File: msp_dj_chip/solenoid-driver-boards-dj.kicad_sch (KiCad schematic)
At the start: 0 parts

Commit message: updated changes
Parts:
- added C19: C_Small, symbol Device:C_Small
- added Q1: NMOS, symbol Simulation_SPICE:NMOS
- added R48: 30K, symbol Device:R_Small
- added R49: 500, symbol Device:R_Small
- added R50: 1K2, symbol Device:R_Small
- added R51, R52: 1, symbol Device:R_Small
- added R53: 0, symbol Device:R_Small
- added TP2, TP3, TP4, TP5, TP6: TestPoint, symbol Connector:TestPoint
- added U16: ${SIM.PARAMS}, symbol Simulation_SPICE:OPAMP
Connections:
- new net: R48.2, R49.1, TP2.1, U16.1 (+)
- new net: C19.2, Q1.2 (G), R51.2, R53.1, TP5.1
- new net: Q1.1 (D), TP6.1
- new net: C19.1, R53.2, U16.5
- new net: Q1.3 (S), R50.1, R50.2, R52.2, TP3.1, TP4.1, U16.2 (-)
- new net +24V: U16.3 (V+)
- new net GND: R49.2, R51.1, R52.1, U16.4 (V-)

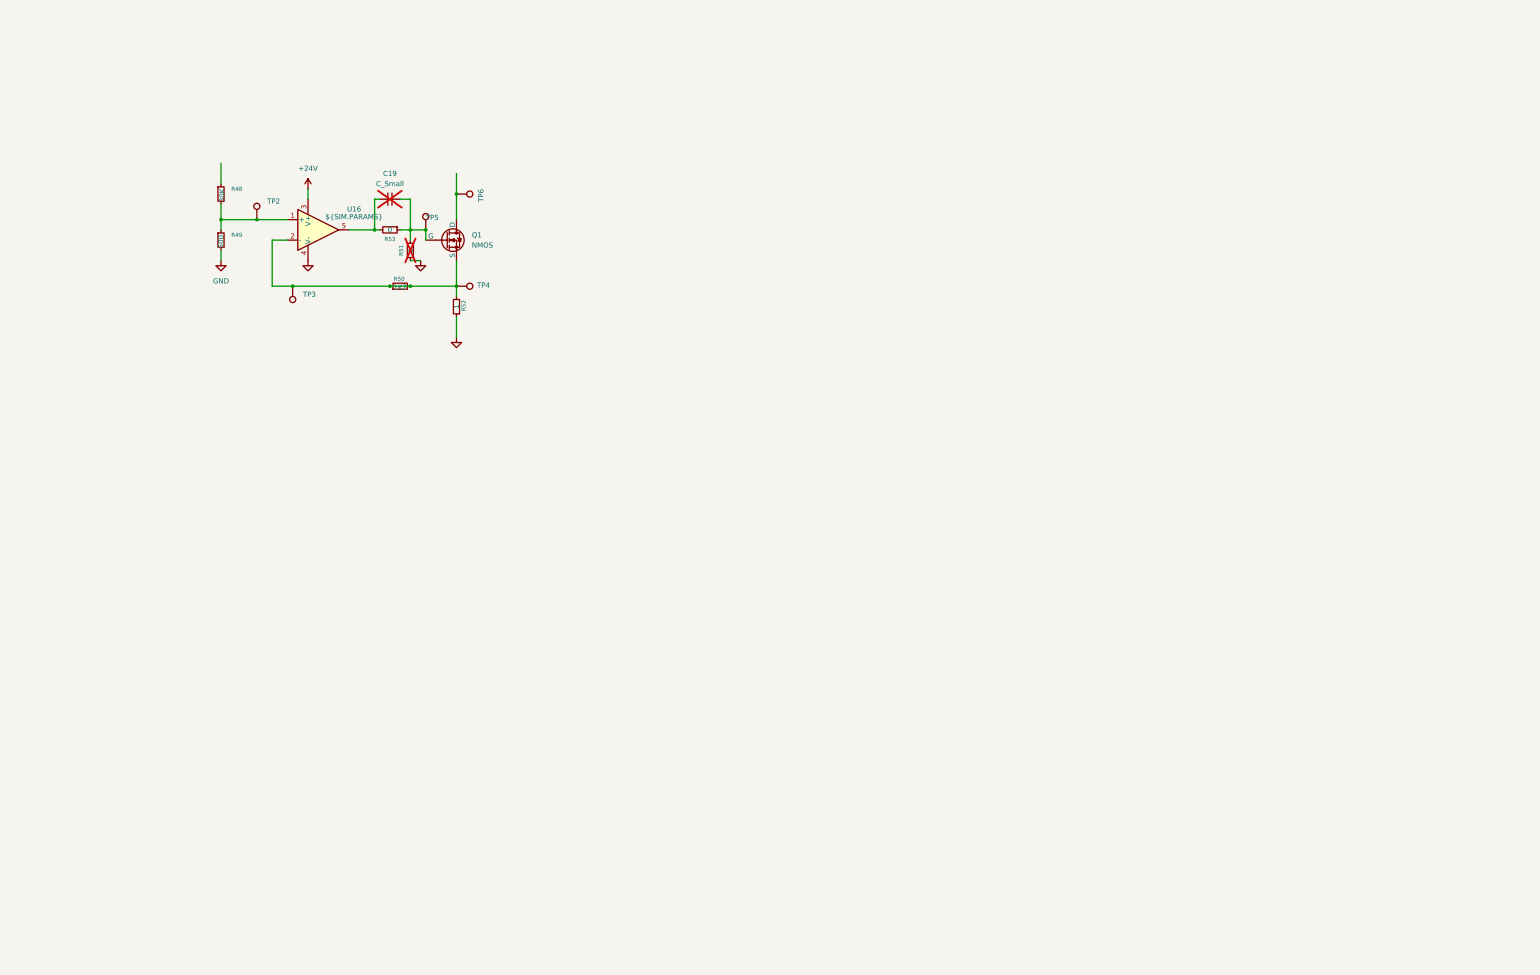
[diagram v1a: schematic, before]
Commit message: SOL-DRIVER-SHEET-ADDED
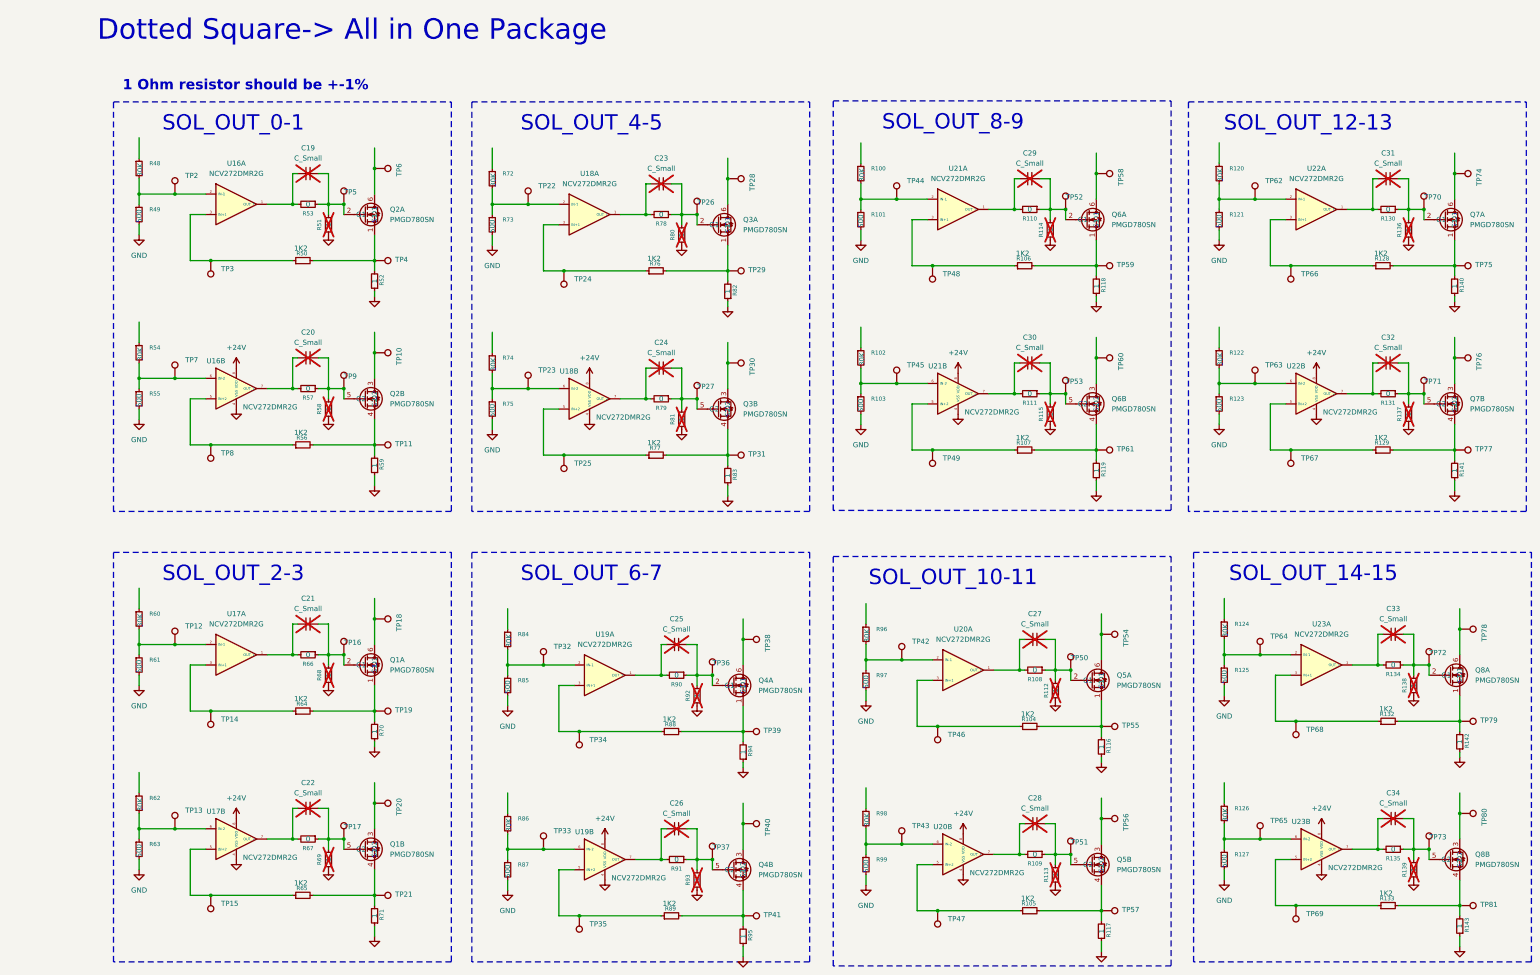
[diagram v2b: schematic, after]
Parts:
- removed Q1: NMOS, symbol Simulation_SPICE:NMOS
- removed U16: ${SIM.PARAMS}, symbol Simulation_SPICE:OPAMP
- added C20, C21, C22, C23, C24, C25, C26, C27, C28, C29, C30, C31, C32, C33, C34: C_Small, symbol Device:C_Small
- added Q1, Q2, Q3, Q4, Q5, Q6, Q7, Q8: PMGD780SN, project_footprints:PMGD780SN, symbol Project_Symbols:2N-Channel_MOSFET
- added R100, R102, R120, R122, R124, R126, R54, R60, R62, R72, R74, R84, R86, R96, R98: 30K, symbol Device:R_Small
- added R101, R103, R121, R123, R125, R127, R55, R61, R63, R73, R75, R85, R87, R97, R99: 500, symbol Device:R_Small
- added R104, R105, R106, R107, R128, R129, R132, R133, R56, R64, R65, R76, R77, R88, R89: 1K2, symbol Device:R_Small
- added R108, R109, R110, R111, R130, R131, R134, R135, R57, R66, R67, R78, R79, R90, R91: 0, symbol Device:R_Small
- added R112, R113, R114, R115, R116, R117, R118, R119, R136, R137, R138, R139, R140, R141, R142, R143, R58, R59, R68, R69, R70, R71, R80, R81, R82, R83, R92, R93, R94, R95: 1, symbol Device:R_Small
- added TP10, TP11, TP12, TP13, TP14, TP15, TP16, TP17, TP18, TP19, TP20, TP21, TP22, TP23, TP24, TP25, TP26, TP27, TP28, TP29, TP30, TP31, TP32, TP33, TP34, TP35, TP36, TP37, TP38, TP39, TP40, TP41, TP42, TP43, TP44, TP45, TP46, TP47, TP48, TP49, TP50, TP51, TP52, TP53, TP54, TP55, TP56, TP57, TP58, TP59, TP60, TP61, TP62, TP63, TP64, TP65, TP66, TP67, TP68, TP69, TP7, TP70, TP71, TP72, TP73, TP74, TP75, TP76, TP77, TP78, TP79, TP8, TP80, TP81, TP9: TestPoint, symbol Connector:TestPoint
- added U16, U17, U18, U19, U20, U21, U22, U23: NCV272DMR2G, Package_SO:MSOP-8_3x3mm_P0.65mm, symbol Project_Symbols:OpAmp_NCV272
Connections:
- net +24V: now also U16.8 (VDD), U17.8 (VDD), U18.8 (VDD), U19.8 (VDD), U20.8 (VDD), U21.8 (VDD), U22.8 (VDD), U23.8 (VDD)
- net GND: now also R101.2, R103.2, R112.1, R113.1, R114.1, R115.1, R116.1, R117.1, R118.1, R119.1, R121.2, R123.2, R125.2, R127.2, R136.1, R137.1, R138.1, R139.1, R140.1, R141.1, R142.1, R143.1, R55.2, R58.1, R59.1, R61.2, R63.2, R68.1, R69.1, R70.1, R71.1, R73.2, R75.2, R80.1, R81.1, R82.1, R83.1, R85.2, R87.2, R92.1, R93.1, R94.1, R95.1, R97.2, R99.2, U16.4 (VSS), U17.4 (VSS), U18.4 (VSS), U19.4 (VSS), U20.4 (VSS), U21.4 (VSS), U22.4 (VSS), U23.4 (VSS)
- net at R48.2, R49.1, TP2.1: now also U16.2 (IN-1)
- net at C19.2, R51.2, R53.1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: now also Q2.2 (G1)
- net at TP6.1: now also Q2.6 (D1)
- net at C19.1, R53.2: now also U16.1 (OUT_1)
- net at R50.2, R52.2, TP4.1: now also Q2.1 (S1); no longer R50.1, TP3.1
- new net: C23.2, Q3.2 (G1), R78.1, R80.2, TP26.1
- new net: R72.2, R73.1, TP22.1, U18.2 (IN-1)
- new net: R60.2, R61.1, TP12.1, U17.2 (IN-1)
- new net: C21.2, Q1.2 (G1), R66.1, R68.2, TP16.1
- new net: C21.1, R66.2, U17.1 (OUT_1)
- new net: Q4.4 (S2), R89.2, R95.2, TP41.1
- new net: R96.2, R97.1, TP42.1, U20.2 (IN-1)
- new net: C26.2, Q4.5 (G2), R91.1, R93.2, TP37.1
- new net: R128.1, TP66.1, U22.3 (IN+1)
- new net: C25.2, Q4.2 (G1), R90.1, R92.2, TP36.1
- new net: Q3.6 (D1), TP28.1
- new net: R74.2, R75.1, TP23.1, U18.6 (IN-2)
- new net: Q1.6 (D1), TP18.1
- new net: C27.2, Q5.2 (G1), R108.1, R112.2, TP50.1
- new net: C27.1, R108.2, U20.1 (OUT_1)
- new net: R129.1, TP67.1, U22.5 (IN+2)
- new net: Q7.4 (S2), R129.2, R141.2, TP77.1
- new net: R105.1, TP47.1, U20.5 (IN+2)
- new net: Q8.1 (S1), R132.2, R142.2, TP79.1
- new net: C33.2, Q8.2 (G1), R134.1, R138.2, TP72.1
- new net: Q8.6 (D1), TP78.1
- new net: R126.2, R127.1, TP65.1, U23.6 (IN-2)
- new net: C25.1, R90.2, U19.1 (OUT_1)
- new net: R133.1, TP69.1, U23.5 (IN+2)
- new net: C34.1, R135.2, U23.7 (OUT_2)
- new net: R84.2, R85.1, TP32.1, U19.2 (IN-1)
- new net: R88.1, TP34.1, U19.3 (IN+1)
- new net: R89.1, TP35.1, U19.5 (IN+2)
- new net: R86.2, R87.1, TP33.1, U19.6 (IN-2)
- new net: C26.1, R91.2, U19.7 (OUT_2)
- new net: C24.1, R79.2, U18.7 (OUT_2)
- new net: C24.2, Q3.5 (G2), R79.1, R81.2, TP27.1
- new net: R107.1, TP49.1, U21.5 (IN+2)
- new net: R102.2, R103.1, TP45.1, U21.6 (IN-2)
- new net: C30.1, R111.2, U21.7 (OUT_2)
- new net: R76.1, TP24.1, U18.3 (IN+1)
- new net: C22.1, R67.2, U17.7 (OUT_2)
- new net: C22.2, Q1.5 (G2), R67.1, R69.2, TP17.1
- new net: C20.2, Q2.5 (G2), R57.1, R58.2, TP9.1
- new net: C20.1, R57.2, U16.7 (OUT_2)
- new net: Q3.1 (S1), R76.2, R82.2, TP29.1
- new net: Q8.3 (D2), TP80.1
- new net: Q8.4 (S2), R133.2, R143.2, TP81.1
- new net: C34.2, Q8.5 (G2), R135.1, R139.2, TP73.1
- new net: Q6.3 (D2), TP60.1
- new net: R104.1, TP46.1, U20.3 (IN+1)
- new net: C23.1, R78.2, U18.1 (OUT_1)
- new net: Q4.1 (S1), R88.2, R94.2, TP39.1
- new net: Q4.6 (D1), TP38.1
- new net: Q5.6 (D1), TP54.1
- new net: Q6.6 (D1), TP58.1
- new net: Q3.3 (D2), TP30.1
- new net: Q3.4 (S2), R77.2, R83.2, TP31.1
- new net: R98.2, R99.1, TP43.1, U20.6 (IN-2)
- new net: R65.1, TP15.1, U17.5 (IN+2)
- new net: R62.2, R63.1, TP13.1, U17.6 (IN-2)
- new net: Q2.3 (D2), TP10.1
- new net: Q1.4 (S2), R65.2, R71.2, TP21.1
- new net: Q7.1 (S1), R128.2, R140.2, TP75.1
- new net: C31.2, Q7.2 (G1), R130.1, R136.2, TP70.1
- new net: Q7.6 (D1), TP74.1
- new net: R100.2, R101.1, TP44.1, U21.2 (IN-1)
- new net: Q1.1 (S1), R64.2, R70.2, TP19.1
- new net: Q5.1 (S1), R104.2, R116.2, TP55.1
- new net: C33.1, R134.2, U23.1 (OUT_1)
- new net: R124.2, R125.1, TP64.1, U23.2 (IN-1)
- new net: R132.1, TP68.1, U23.3 (IN+1)
- new net: R77.1, TP25.1, U18.5 (IN+2)
- new net: R106.1, TP48.1, U21.3 (IN+1)
- new net: C30.2, Q6.5 (G2), R111.1, R115.2, TP53.1
- new net: R56.1, TP8.1, U16.5 (IN+2)
- new net: Q2.4 (S2), R56.2, R59.2, TP11.1
- new net: R120.2, R121.1, TP62.1, U22.2 (IN-1)
- new net: C31.1, R130.2, U22.1 (OUT_1)
- new net: Q6.1 (S1), R106.2, R118.2, TP59.1
- new net: C29.2, Q6.2 (G1), R110.1, R114.2, TP52.1
- new net: Q4.3 (D2), TP40.1
- new net: Q5.3 (D2), TP56.1
- new net: Q5.4 (S2), R105.2, R117.2, TP57.1
- new net: C28.2, Q5.5 (G2), R109.1, R113.2, TP51.1
- new net: R122.2, R123.1, TP63.1, U22.6 (IN-2)
- new net: R54.2, R55.1, TP7.1, U16.6 (IN-2)
- new net: R50.1, TP3.1, U16.3 (IN+1)
- new net: Q6.4 (S2), R107.2, R119.2, TP61.1
- new net: R64.1, TP14.1, U17.3 (IN+1)
- new net: C29.1, R110.2, U21.1 (OUT_1)
- new net: Q7.3 (D2), TP76.1
- new net: C32.2, Q7.5 (G2), R131.1, R137.2, TP71.1
- new net: C32.1, R131.2, U22.7 (OUT_2)
- new net: C28.1, R109.2, U20.7 (OUT_2)
- new net: Q1.3 (D2), TP20.1
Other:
- note added: "1 Ohm resistor should be +-1%"
- note added: "Dotted Square-> All in One Package"
- note added: "SOL_OUT_0-1"
- note added: "SOL_OUT_10-11"
- note added: "SOL_OUT_12-13"
- note added: "SOL_OUT_14-15"
- note added: "SOL_OUT_2-3"
- note added: "SOL_OUT_4-5"
- note added: "SOL_OUT_6-7"
- note added: "SOL_OUT_8-9"
- moved on the sheet: C19, R48, R49, R50, R51, R52, R53, TP2, TP3, TP4, TP5, TP6
